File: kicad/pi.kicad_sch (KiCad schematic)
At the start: 23 parts, among them J5 SWD, M2 Fan_4pin, P2 MYUSB_B, U13 TMP1075, U3 STM32L052K6Tx

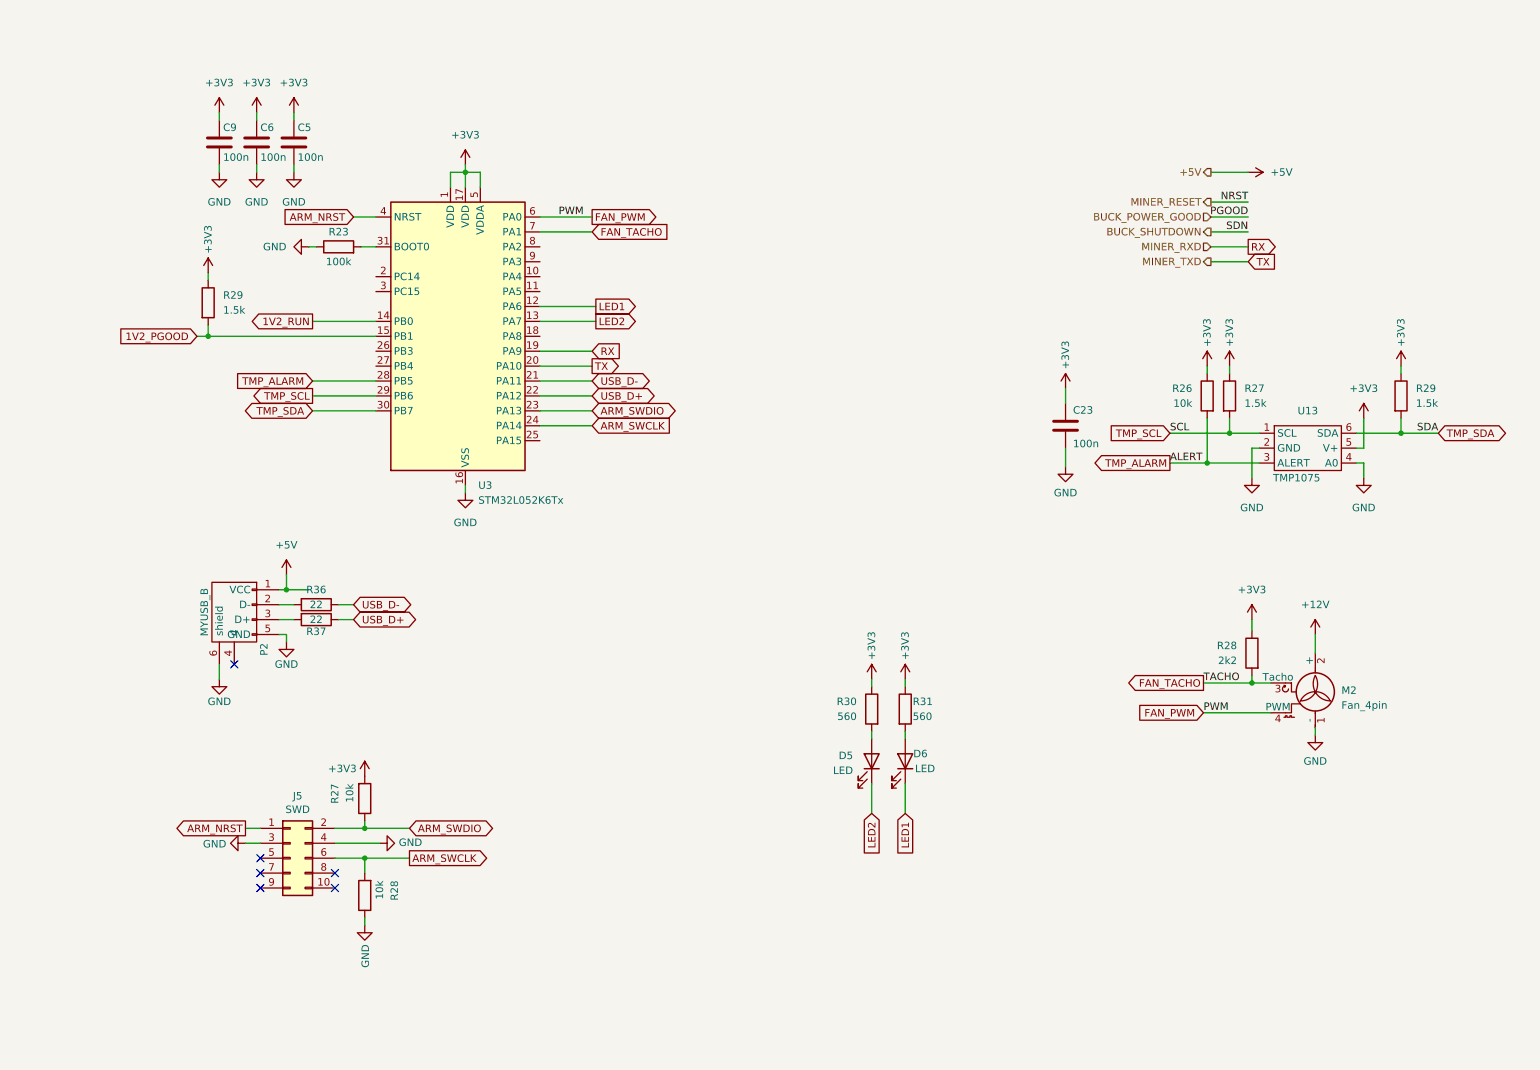
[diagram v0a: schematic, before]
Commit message: updated gerber, bom
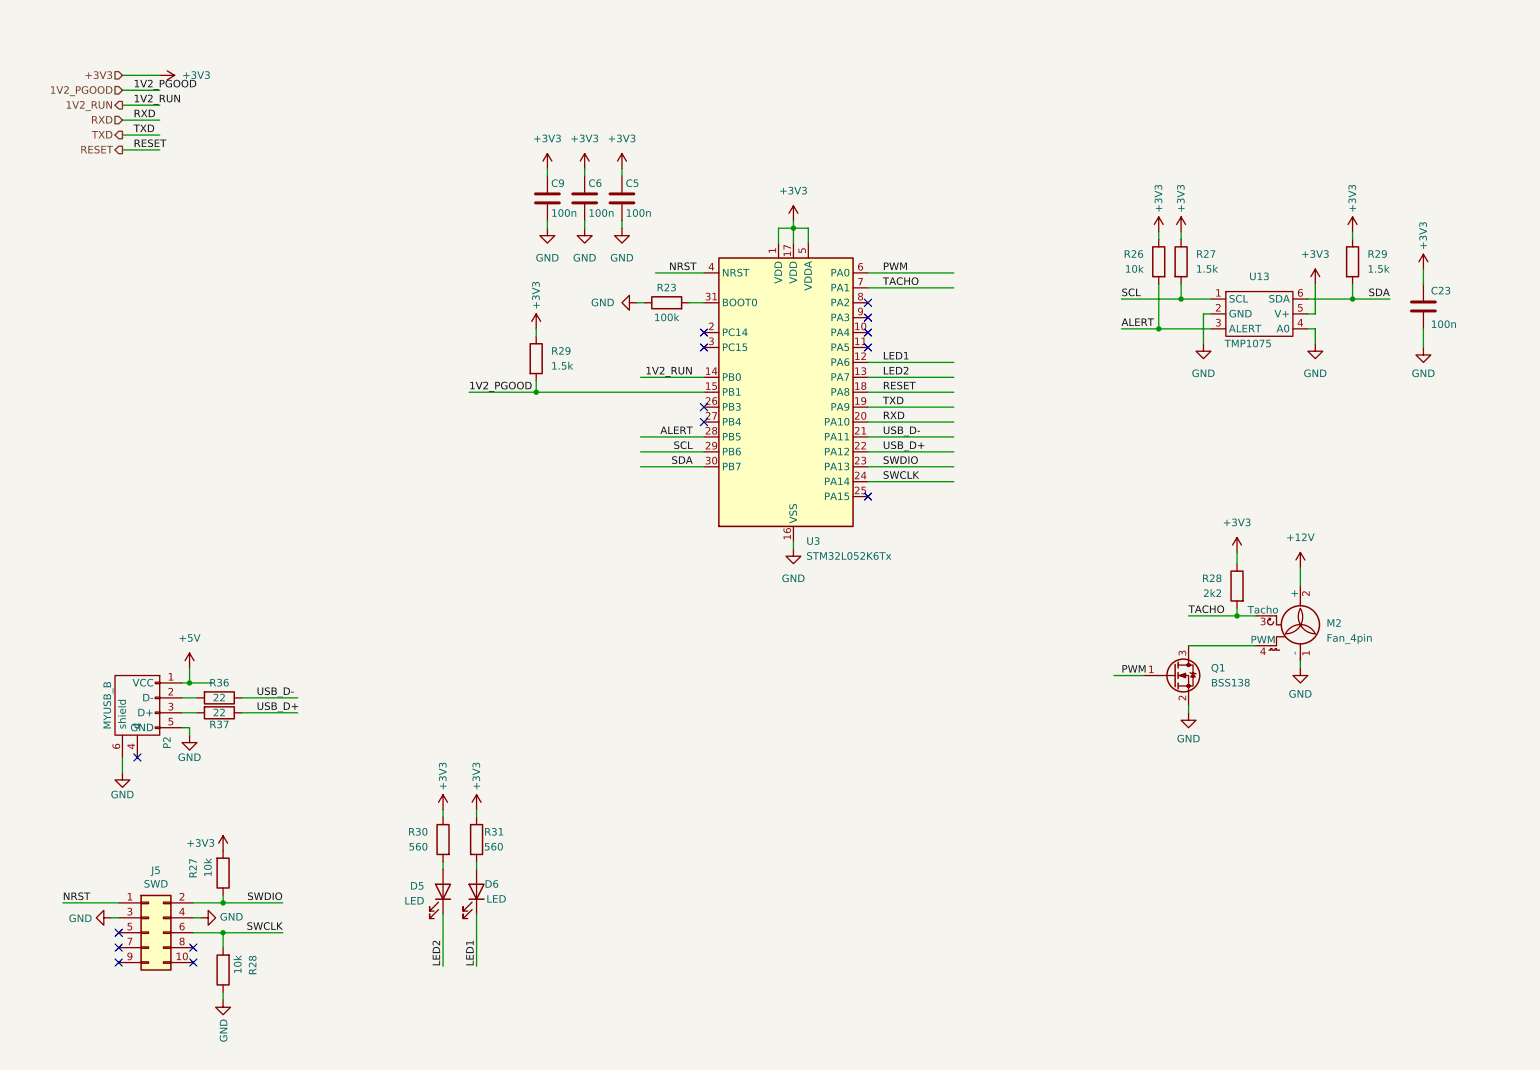
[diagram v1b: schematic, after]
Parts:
- added Q1: BSS138, Package_TO_SOT_SMD:SOT-23, symbol Transistor_FET:BSS138
- C23: PARTNO 0402X104K100CT -> (none)
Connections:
- net GND: now also Q1.2 (S)
- net RESET: now reaches U3.18 (PA8)
- net ARM_NRST renamed NRST
- net ARM_SWCLK renamed SWCLK
- net ARM_SWDIO renamed SWDIO
- net FAN_PWM: no longer names the net of M2.4 (PWM)
- net FAN_PWM: now also Q1.3 (D); no longer U3.6 (PA0)
- net FAN_TACHO renamed TACHO
- net RX renamed TXD
- net TMP_ALARM renamed ALERT
- net TMP_SCL renamed SCL
- net TMP_SDA renamed SDA
- net TX renamed RXD
- new net PWM: Q1.1 (G), U3.6 (PA0)
- no-connect marks 6 -> 15
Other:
- moved on the sheet: C23, C5, C6, C9, D5, D6, J5, M2, P2, R23, R26, R27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

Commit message: v0.02
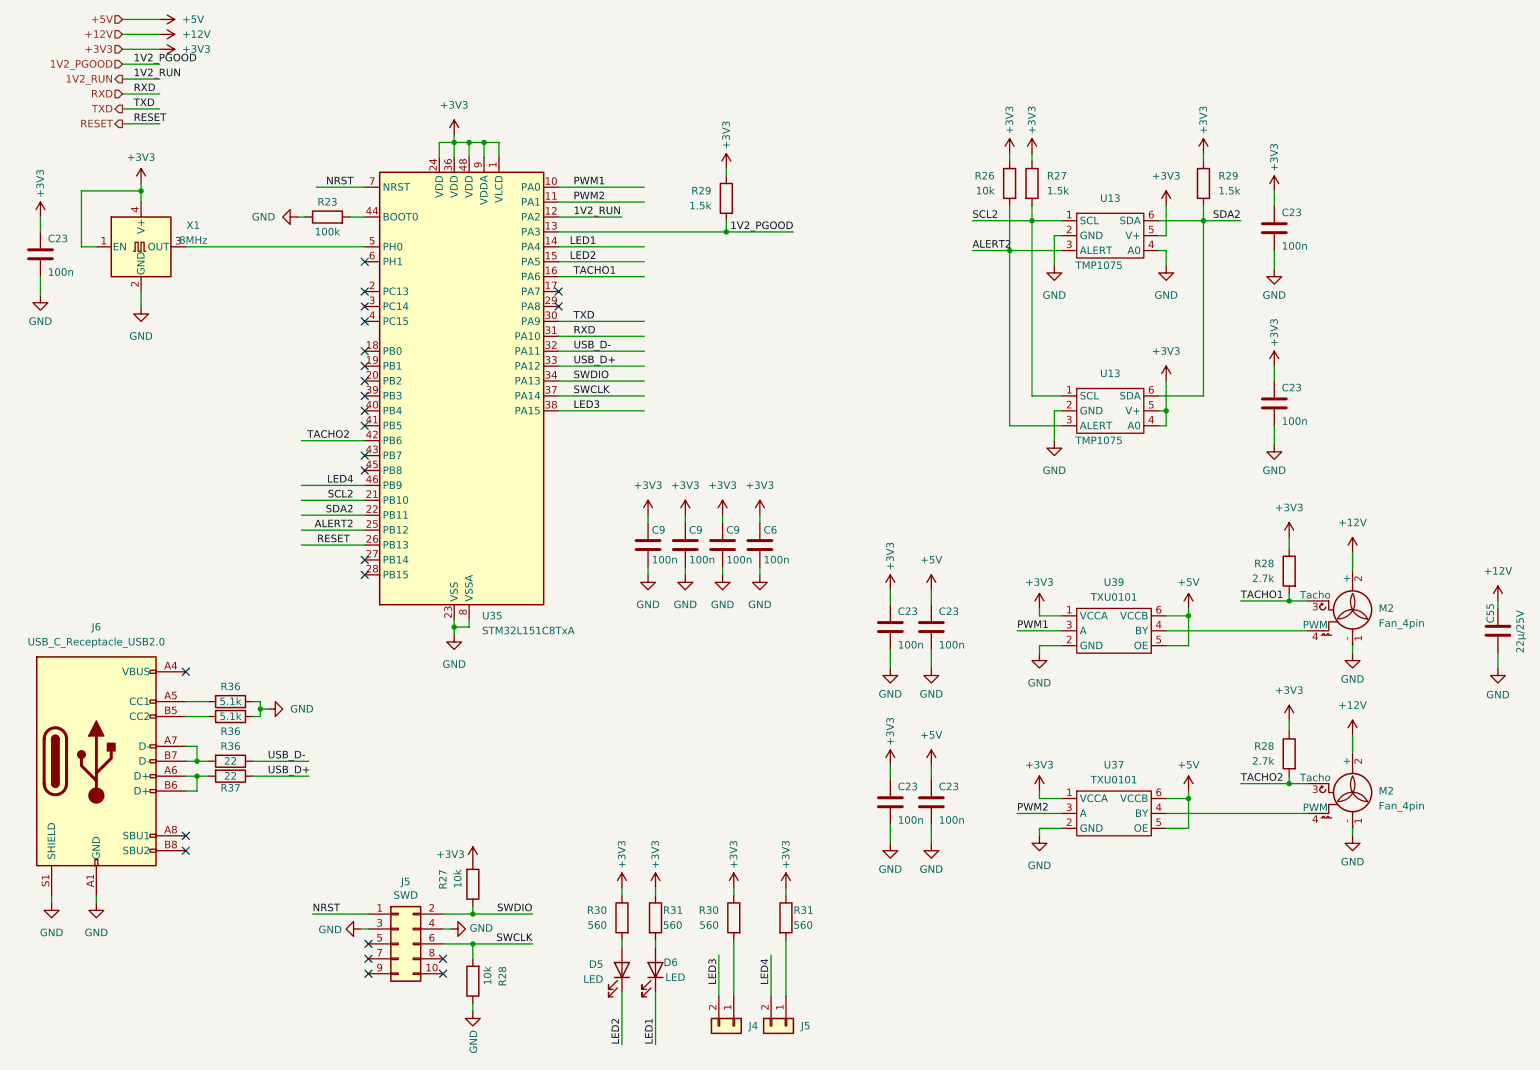
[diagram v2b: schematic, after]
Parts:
- removed C5: 100n, Capacitor_SMD:C_0805_2012Metric, symbol vfd1-rescue:C
- removed P2: MYUSB_B, Connector_USB:USB_Micro-B_Amphenol_10103594-0001LF_Horizontal, symbol clock-rescue:MYUSB_B
- removed Q1: BSS138, Package_TO_SOT_SMD:SOT-23, symbol Transistor_FET:BSS138
- removed U3: STM32L052K6Tx, Package_QFP:LQFP-32_7x7mm_P0.8mm, symbol MCU_ST_STM32L0:STM32L052K6Tx
- added C23 (x6): 100n, Capacitor_SMD:C_0805_2012Metric, symbol Device:C
- added C55: 22µ/25V, Capacitor_SMD:C_1210_3225Metric, symbol Device:C
- added C9 (x2): 100n, Capacitor_SMD:C_0805_2012Metric, symbol vfd1-rescue:C
- added J4, J5: Conn_01x02, Connector_PinHeader_2.54mm:PinHeader_1x02_P2.54mm_Vertical, symbol Connector_Generic:Conn_01x02
- added J6: USB_C_Receptacle_USB2.0, Connector_USB:USB_C_Receptacle_GCT_USB4105-xx-A_16P_TopMnt_Horizontal, symbol Connector:USB_C_Receptacle_USB2.0
- added M2: Fan_4pin, Connector:FanPinHeader_1x04_P2.54mm_Vertical, symbol Motor:Fan_4pin
- added R28: 2.7k, Resistor_SMD:R_0805_2012Metric, symbol Device:R
- added R30, R31: 560, Resistor_SMD:R_0805_2012Metric, symbol Device:R
- added R36 (x2): 5.1k, Resistor_SMD:R_0805_2012Metric, symbol clock-rescue:R
- added U13: TMP1075, myfootprints:TMP1075-DRL, symbol mylib7:TMP1075-DRL-SOT563
- added U35: STM32L151C8TxA, Package_QFP:LQFP-48_7x7mm_P0.5mm, symbol MCU_ST_STM32L1:STM32L151C8TxA
- added U37, U39: TXU0101, Package_TO_SOT_SMD:SOT-363_SC-70-6, symbol mylib7:TXU0101DCK
- added X1: 8MHz, Oscillator:Oscillator_SMD_EuroQuartz_XO32-4Pin_3.2x2.5mm, symbol Oscillator:XO32
- R28: value 2k2 -> 2.7k
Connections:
- net +12V: now also C55.1, M2.2 (+)
- net +3V3: now also C23.1, C23.1, C23.1, C23.1, C9.1, C9.1, R28.1, R30.1, R31.1, U13.4 (A0), U13.5 (V+), U35.1 (VLCD), U35.24 (VDD), U35.36 (VDD), U35.48 (VDD), U35.9 (VDDA), U37.1 (VCCA), U39.1 (VCCA), X1.1 (EN), X1.4 (V+)
- net +5V: now also C23.1, C23.1, U37.5 (OE), U37.6 (VCCB), U39.5 (OE), U39.6 (VCCB)
- net 1V2_PGOOD: now also U35.13 (PA3)
- net 1V2_RUN: now also U35.12 (PA2)
- net GND: now also C23.2, C23.2, C23.2, C23.2, C23.2, C23.2, C55.2, C9.2, C9.2, J6.A1 (GND), J6.A12 (GND), J6.B1 (GND), J6.B12 (GND), J6.S1 (SHIELD), M2.1 (-), R36.1, R36.1, U13.2 (GND), U35.23 (VSS), U35.35 (VSS), U35.47 (VSS), U35.8 (VSSA), U37.2 (GND), U39.2 (GND), X1.2 (GND)
- net LED1: now also U35.14 (PA4)
- net LED2: now also U35.15 (PA5)
- net NRST: now also U35.7 (NRST)
- net RESET: now also U35.26 (PB13)
- net RXD: now also U35.31 (PA10)
- net SWCLK: now also U35.37 (PA14)
- net SWDIO: now also U35.34 (PA13)
- net TXD: now also U35.30 (PA9)
- net USB_D+: now also U35.33 (PA12)
- net USB_D-: now also U35.32 (PA11)
- net at R36.2: now also J6.A7 (D-), J6.B7 (D-)
- net at R37.2: now also J6.A6 (D+), J6.B6 (D+)
- net at M2.4 (PWM): now also U39.4 (BY)
- net at R23.2: now also U35.44 (BOOT0)
- net ALERT renamed ALERT2
- net ALERT2: now also U13.3 (ALERT), U35.25 (PB12)
- net SCL renamed SCL2
- net SCL2: now also U13.1 (SCL), U35.21 (PB10)
- net SDA renamed SDA2
- net SDA2: now also U13.6 (SDA), U35.22 (PB11)
- net TACHO renamed TACHO1
- net TACHO1: now also U35.16 (PA6)
- new net: M2.4 (PWM), U37.4 (BY)
- new net: J5.1 (Pin_1), R31.2
- new net: J6.A5 (CC1), R36.2
- new net: J4.1 (Pin_1), R30.2
- new net: U35.5 (PH0), X1.3 (OUT)
- new net: J6.B5 (CC2), R36.2
- new net: J6.A4 (VBUS), J6.A9 (VBUS), J6.B4 (VBUS), J6.B9 (VBUS)
- new net LED3: J4.2 (Pin_2), U35.38 (PA15)
- new net LED4: J5.2 (Pin_2), U35.46 (PB9)
- new net PWM1: U35.10 (PA0), U39.3 (A)
- new net PWM2: U35.11 (PA1), U37.3 (A)
- new net TACHO2: M2.3 (Tacho), R28.2, U35.42 (PB6)
- no-connect marks 15 -> 24
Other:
- moved on the sheet: C23, C6, C9, D5, D6, J5, M2, R23, R26, R27, R28, R29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
